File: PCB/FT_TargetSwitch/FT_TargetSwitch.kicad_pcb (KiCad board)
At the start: 2 copper layers, 73 x 73 mm, 11 parts

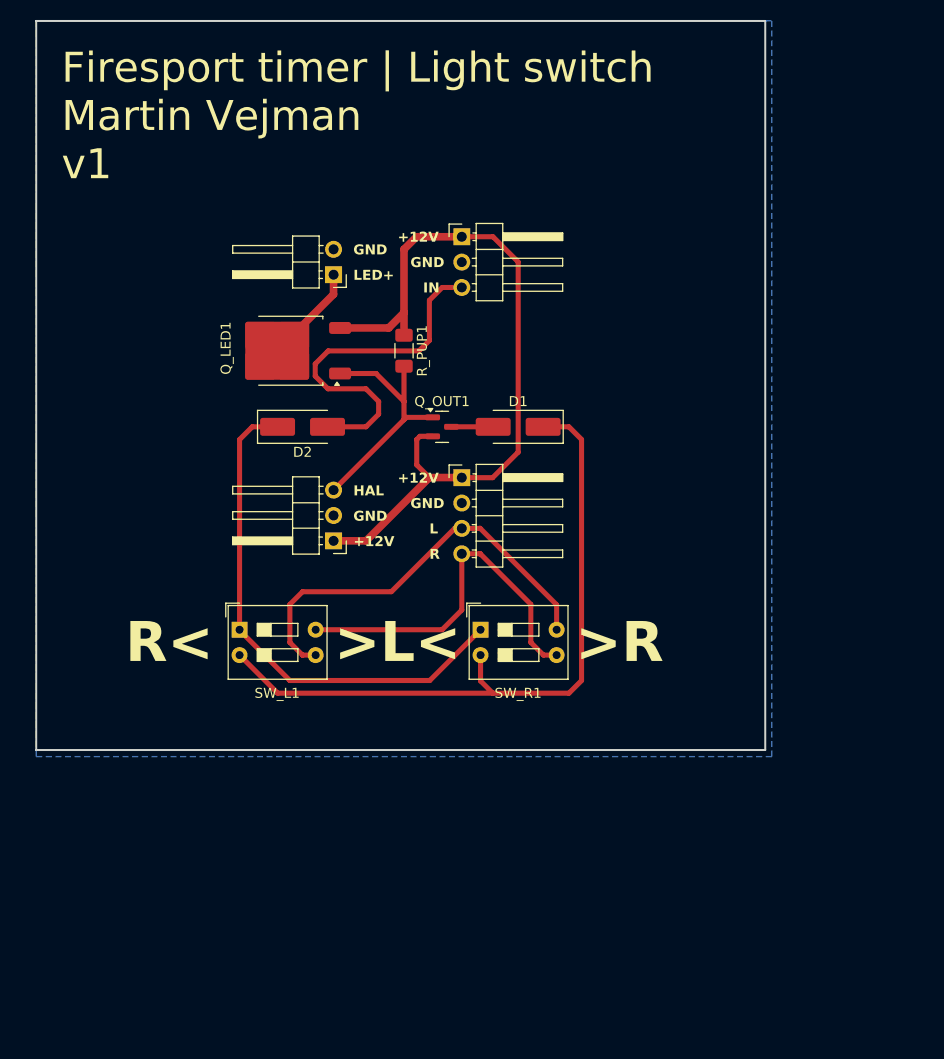
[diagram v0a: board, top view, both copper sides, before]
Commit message: update pcbs
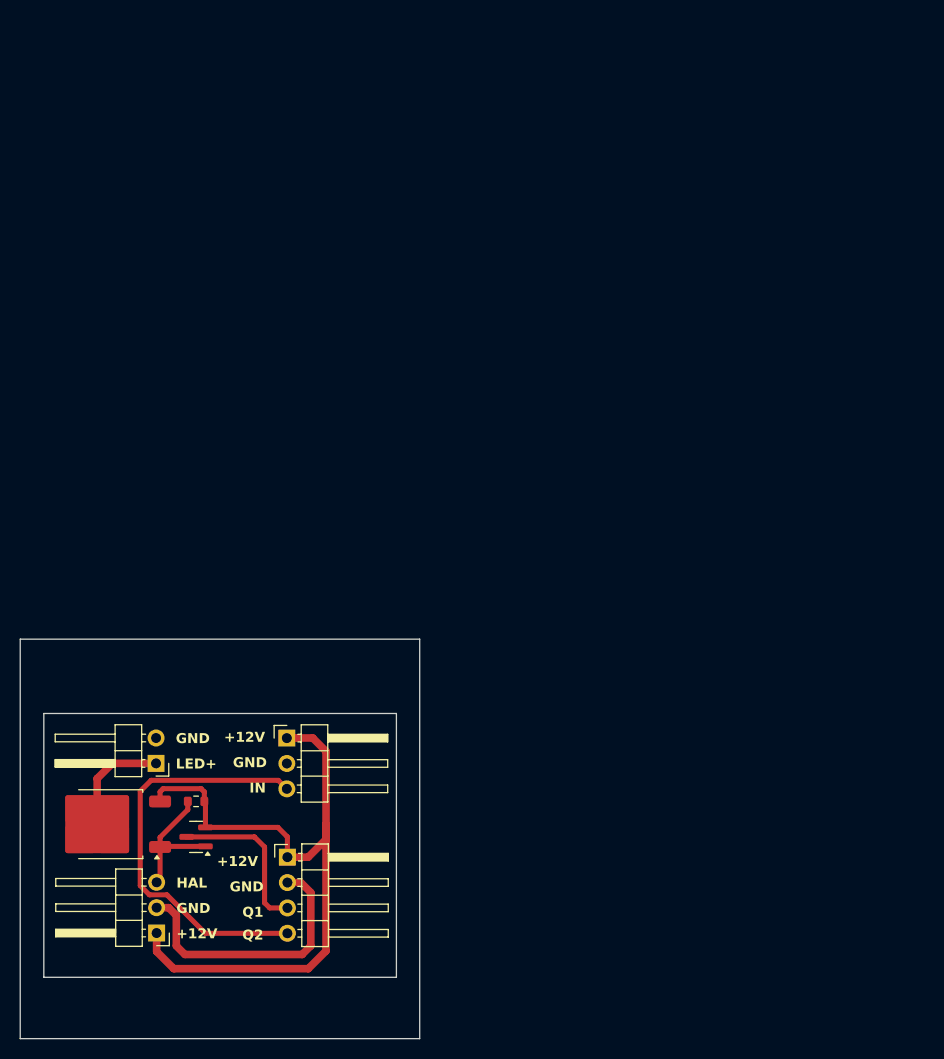
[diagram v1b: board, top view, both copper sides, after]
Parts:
- removed D1, D2: M7, Diode_SMD:D_SMA_Handsoldering
- removed SW_L1, SW_R1: SW_DIP_x02, Button_Switch_THT:SW_DIP_SPSTx02_Slide_9.78x7.26mm_W7.62mm_P2.54mm
- R_PUP1: footprint Resistor_SMD:R_1206_3216Metric_Pad1.30x1.75mm_HandSolder -> Resistor_SMD:R_0603_1608Metric
- moved CON_PASTHRU1 53.2 mm to (126.7, 109.9)
- moved CON_LED1 52.1 mm to (113.6, 112.4)
- moved Q_LED1 50.7 mm to (109.0, 118.5)
- moved R_PUP1 49.7 mm to (117.6, 116.2), turned to 180 degrees
- moved Q_OUT1 47.9 mm to (117.6, 119.8), turned to 180 degrees
- moved CON_HAL1 43.1 mm to (113.7, 129.4)
- moved CON_IO1 41.8 mm to (126.8, 121.8)
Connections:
- CON_IO1 pad 3: /L_OUT -> /OUT
- CON_IO1 pad 4: /R_OUT -> /PASSTHRU_OUT
- CON_PASTHRU1 pad 3: /PASTRHRU_IN -> /PASSTHRU_OUT
- Q_OUT1 pad 3: /Q_UOT_DRAIN -> /OUT
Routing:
- net /OUT: track 69.3 -> 16.3 mm
- net /PASTHRU_OUT: track 51.7 -> 0.00 mm
- net /L_OUT: track 42.5 -> 0.00 mm
- net /PASSTHRU_OUT: track 0.00 -> 41.6 mm
- net /R_OUT: track 37.1 -> 0.00 mm
- net /PASTRHRU_IN: track 35.7 -> 0.00 mm
- net GND: track 0.00 -> 27.6 mm
- net /HAL_IN: track 25.9 -> 14.0 mm
- net +12V: track 75.9 -> 70.8 mm
- net /Q_UOT_DRAIN: track 4.18 -> 0.00 mm
- net /LED_OUT: track 9.95 -> 11.1 mm
- removed copper zone on B.Cu, net GND
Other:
- board size 73 x 73 mm -> 40 x 40 mm
- board text added: "Q1"
- board text added: "Q2"
- board text removed: ">L<"
- board text removed: ">R"
- board text removed: "Firesport timer | Light switch Martin Vejman v1"
- board text removed: "L"
- board text removed: "R"
- board text removed: "R<"
